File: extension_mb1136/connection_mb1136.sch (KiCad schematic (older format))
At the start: 6 parts, among them CN1 Conn_02x19_Odd_Even, CN2 Conn_02x19_Odd_Even, CN3 Conn_01x08, CN4 Conn_01x06, CN5 Conn_01x08, CN6 Conn_01x10

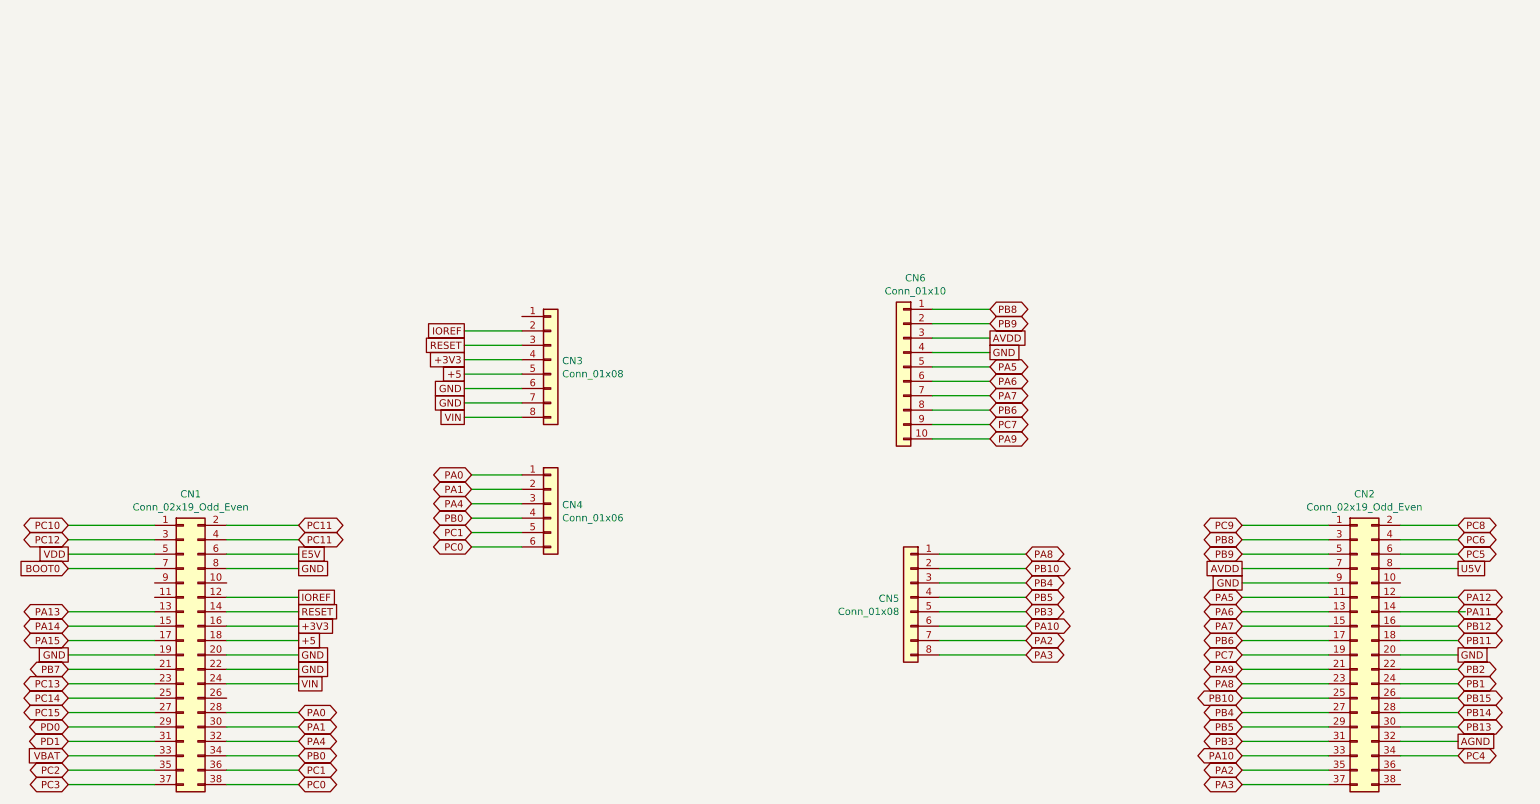
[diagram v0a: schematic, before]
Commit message: update schema
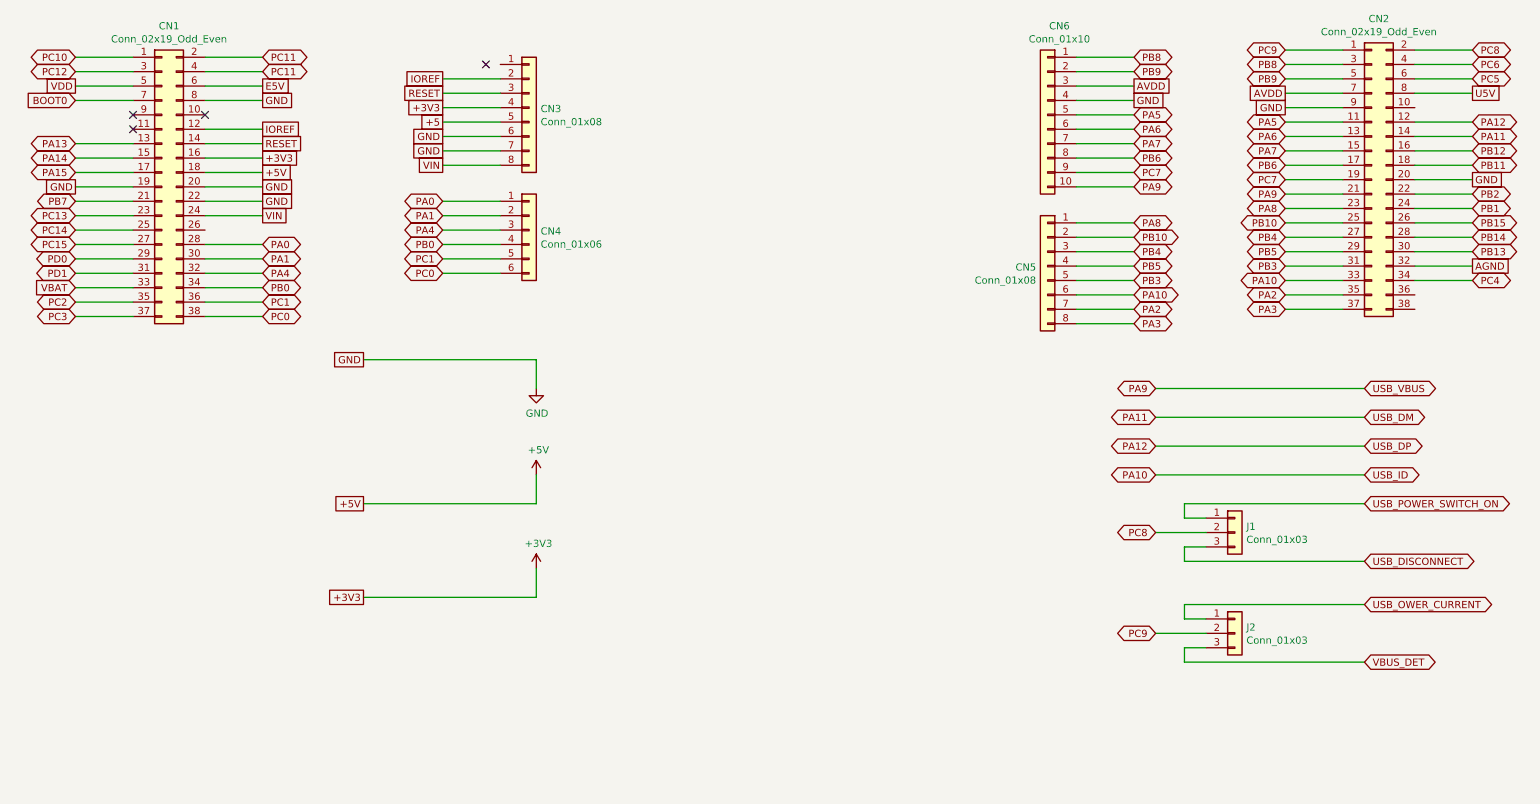
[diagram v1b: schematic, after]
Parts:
- added J1, J2: Conn_01x03, Connector_PinHeader_2.54mm:PinHeader_1x03_P2.54mm_Vertical, symbol Connector_Generic:Conn_01x03
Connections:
- net +5: no longer CN1.18 (Pin_18)
- net PC8: now also J1.2 (Pin_2)
- net PC9: now also J2.2 (Pin_2)
- new net +5V: CN1.18 (Pin_18)
- new net USB_DISCONNECT: J1.3 (Pin_3)
- new net USB_OWER_CURRENT: J2.1 (Pin_1)
- new net USB_POWER_SWITCH_ON: J1.1 (Pin_1)
- new net VBUS_DET: J2.3 (Pin_3)
- no-connect marks 0 -> 4
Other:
- moved on the sheet: CN1, CN2, CN3, CN4, CN5, CN6
